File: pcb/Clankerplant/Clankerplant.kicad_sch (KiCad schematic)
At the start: 31 parts, among them J1 flash, J3 LCD screen, J4 water pump, Q2 AO3400A (mosfet), U1 BQ24074RGTR, U2 ESP32-S3, U3 TPS63900DSKR, Y1 40MHz

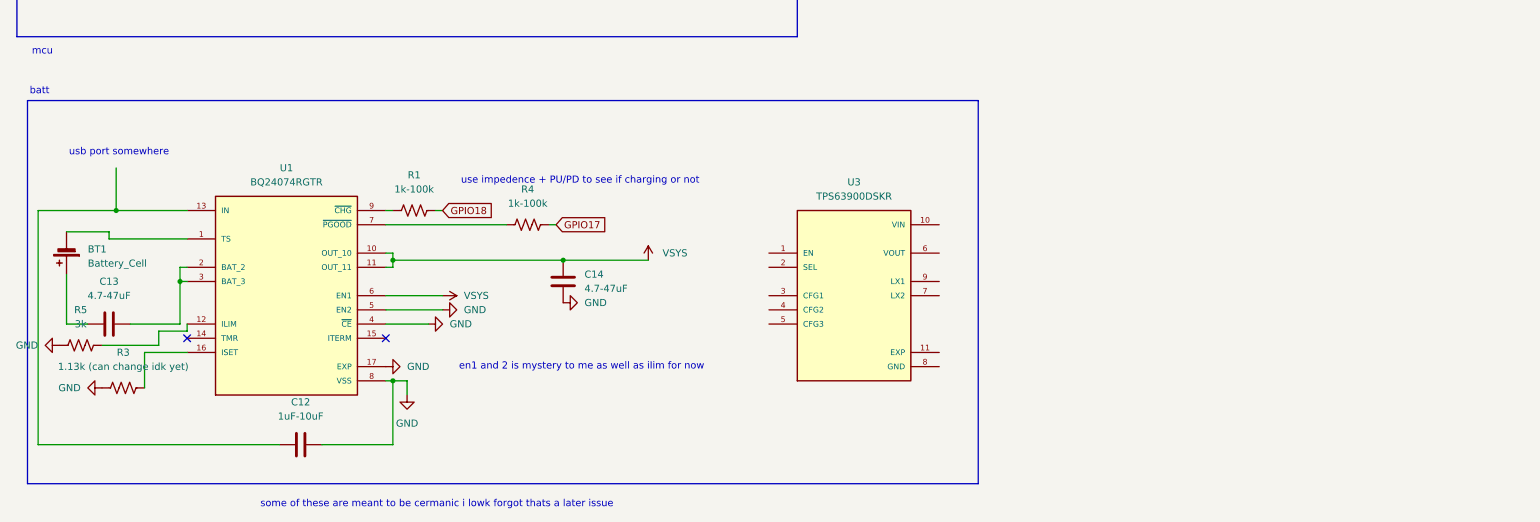
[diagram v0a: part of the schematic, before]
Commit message: 4th of july again
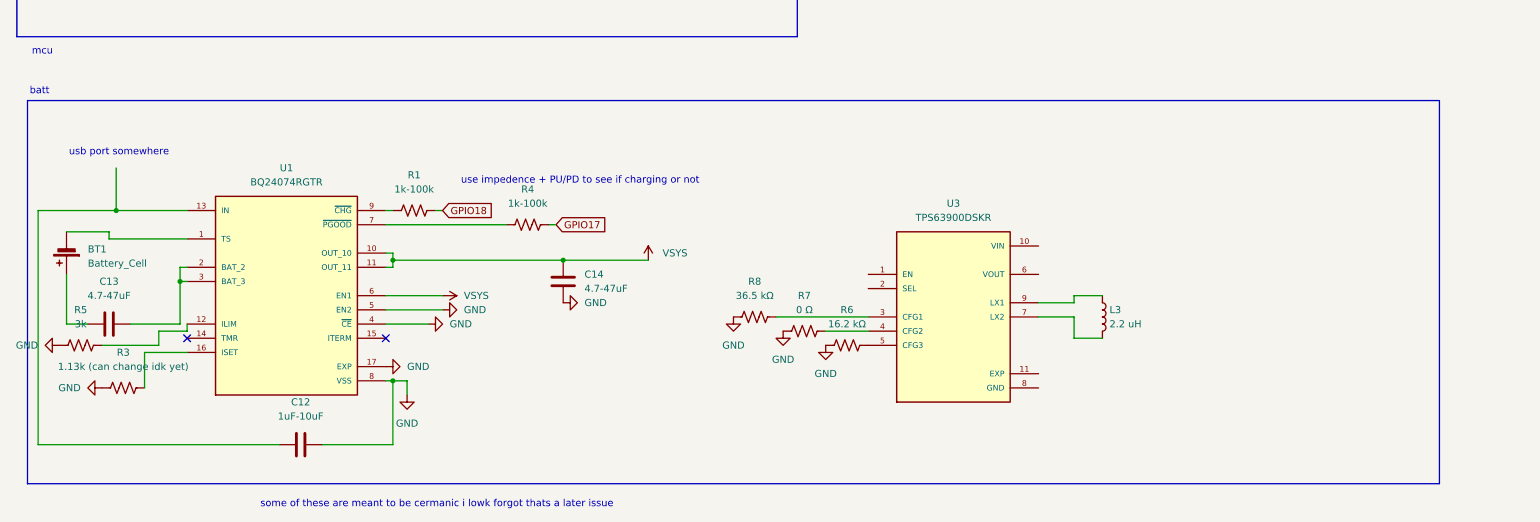
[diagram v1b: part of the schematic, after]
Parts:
- added L3: 2.2 uH, symbol Device:L
- added R6: 16.2 kΩ, symbol Device:R_US
- added R7: 0 Ω, symbol Device:R_US
- added R8: 36.5 kΩ, symbol Device:R_US
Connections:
- net GND: now also R6.2, R7.1, R8.1
- net at U3.3 (CFG1): now also R8.2
- net at U3.4 (CFG2): now also R7.2
- net at U3.5 (CFG3): now also R6.1
- net at U3.7 (LX2): now also L3.2
- net at U3.9 (LX1): now also L3.1
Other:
- note removed: "en1 and 2 is mystery to me as well as ilim for now"
- moved on the sheet: U3
